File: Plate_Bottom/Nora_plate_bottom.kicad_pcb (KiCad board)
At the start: 2 copper layers, 285 x 94.6 mm, 10 parts

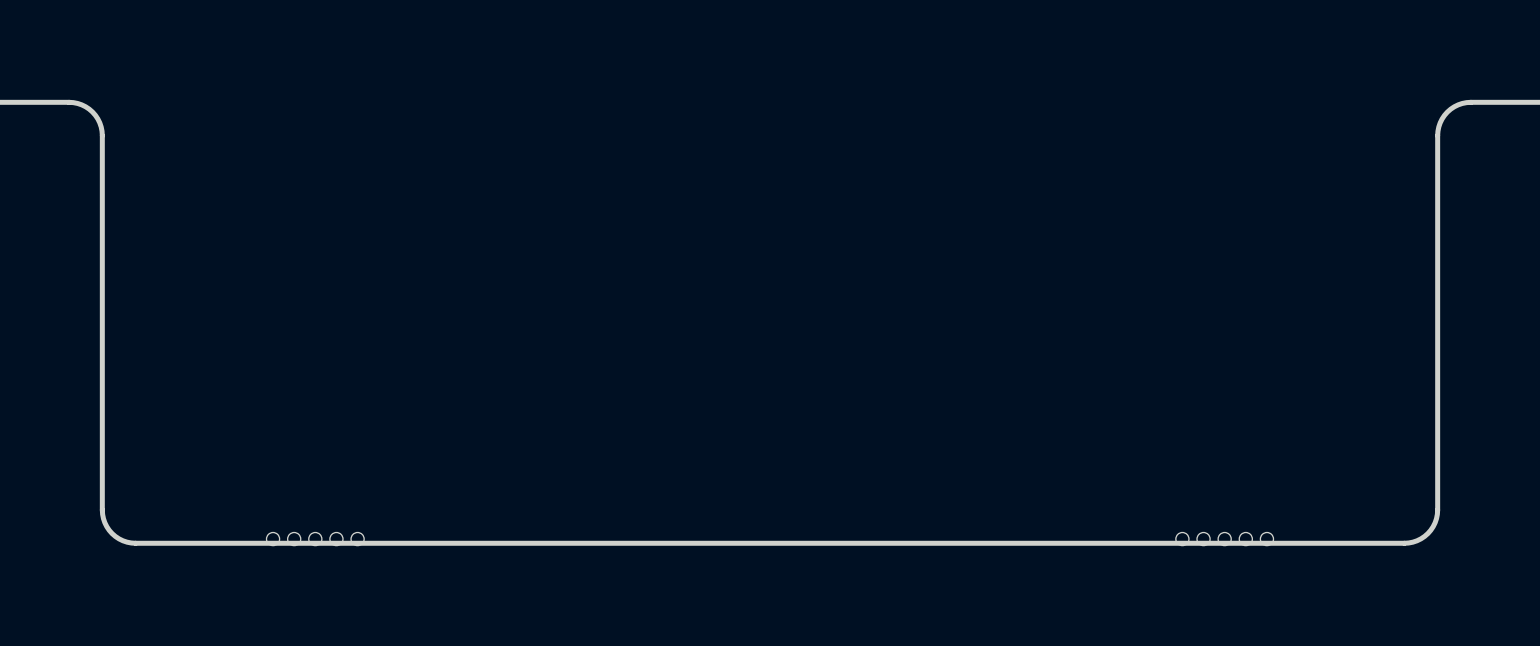
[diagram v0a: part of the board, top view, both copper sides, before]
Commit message: WIP ボトムプレートに切り取りをつけ、さらに改造中
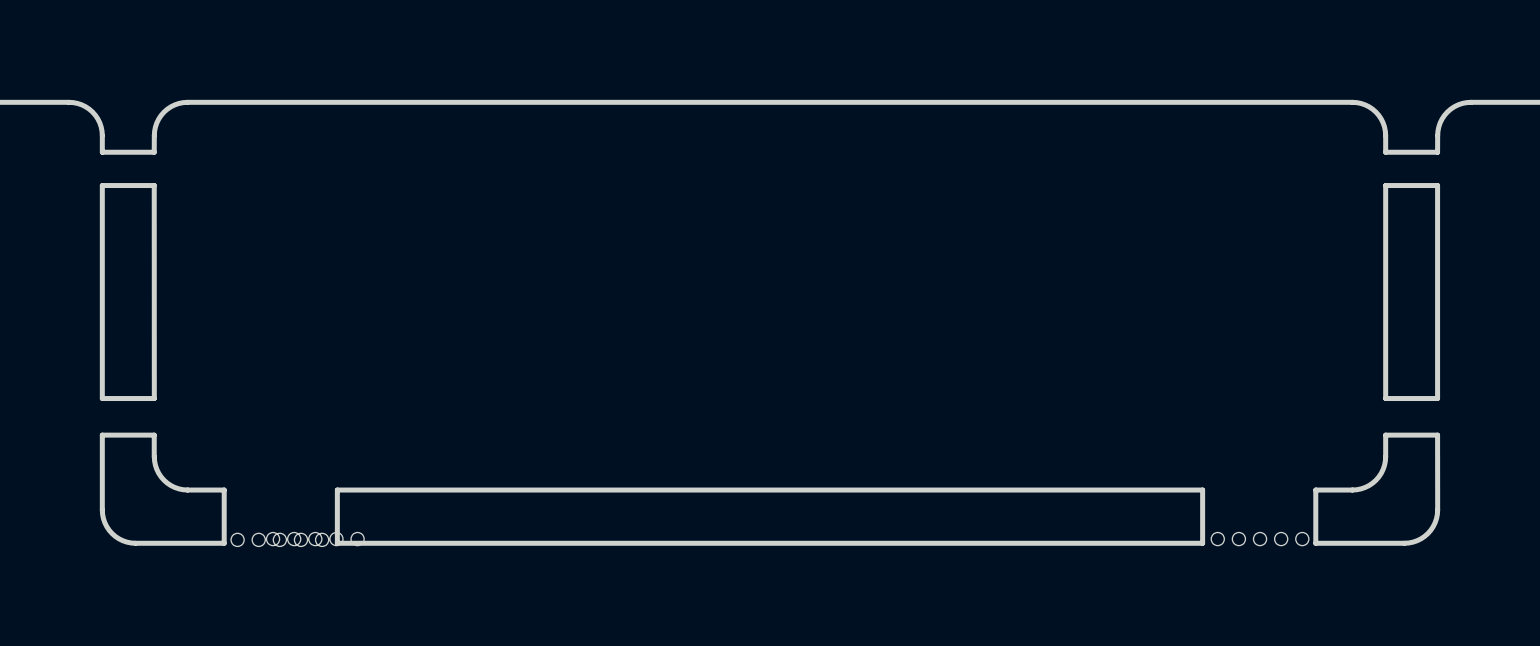
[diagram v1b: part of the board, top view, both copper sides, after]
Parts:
- removed the REF** at (185.2, 43.6)
- REF**: footprint locallib:60_Outline_for_Bottom_USB_cutout_slit_closed_with_PICO -> locallib:60_Outline_Nora_with_PICO_
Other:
- outline, holes or cut-outs redrawn
